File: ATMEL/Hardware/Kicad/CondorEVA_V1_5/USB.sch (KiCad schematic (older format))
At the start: 21 parts, among them J901 USB_2, X901 MINI-USB-32005-201

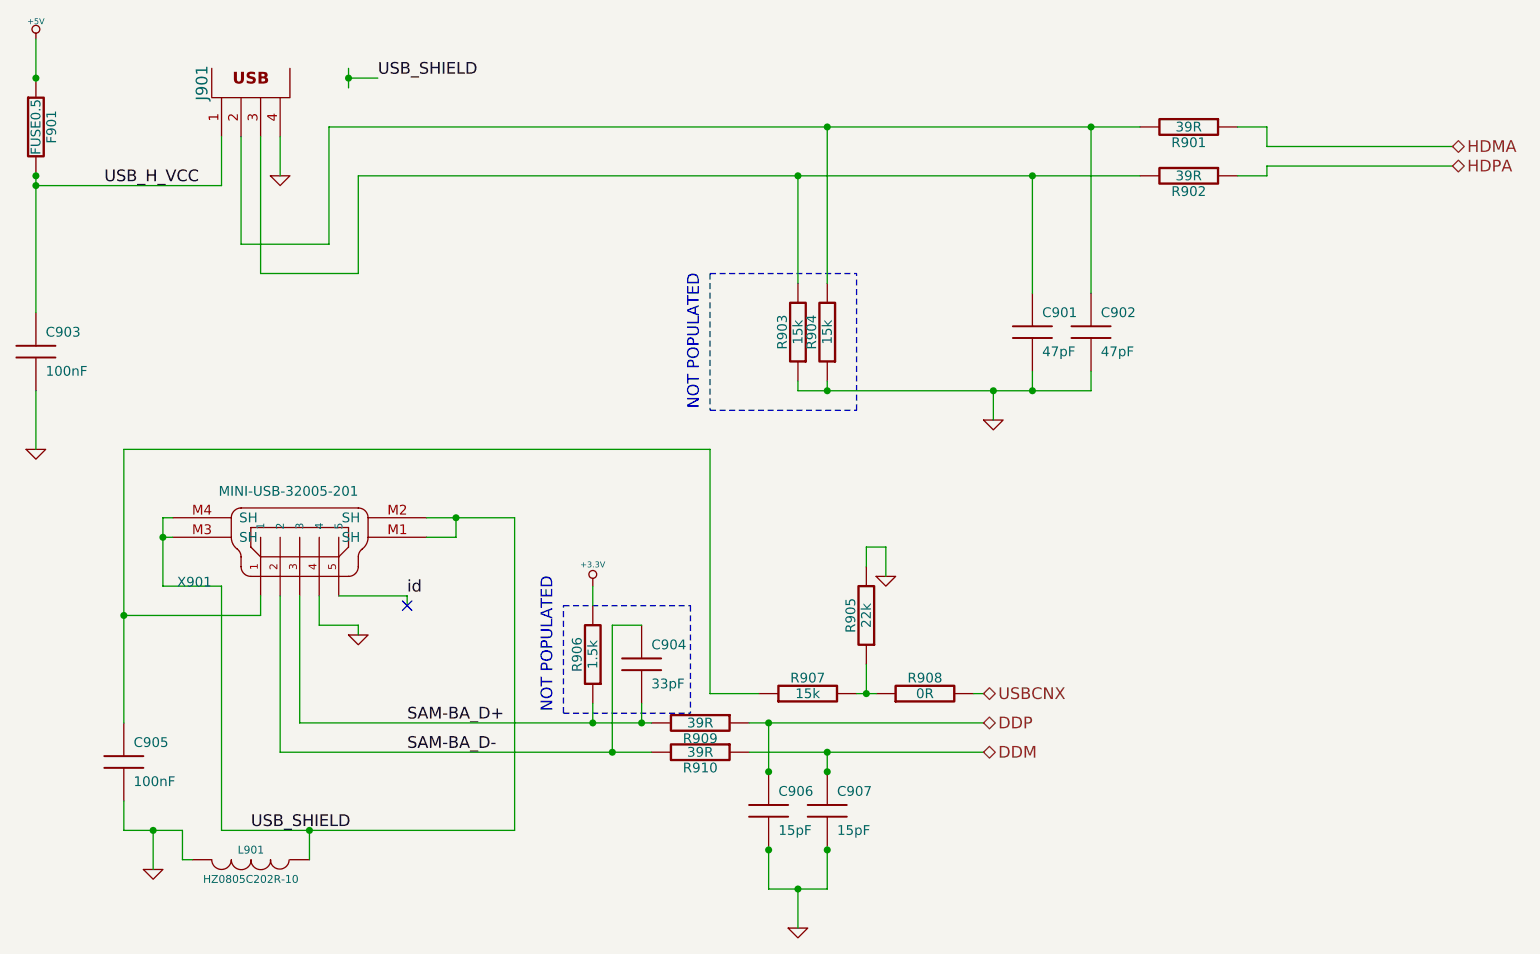
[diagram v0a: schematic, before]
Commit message: Actualización para fabricación lafci Uniandes Enero 19. Orden radicada archivo Ene19.zip con los archivos listos
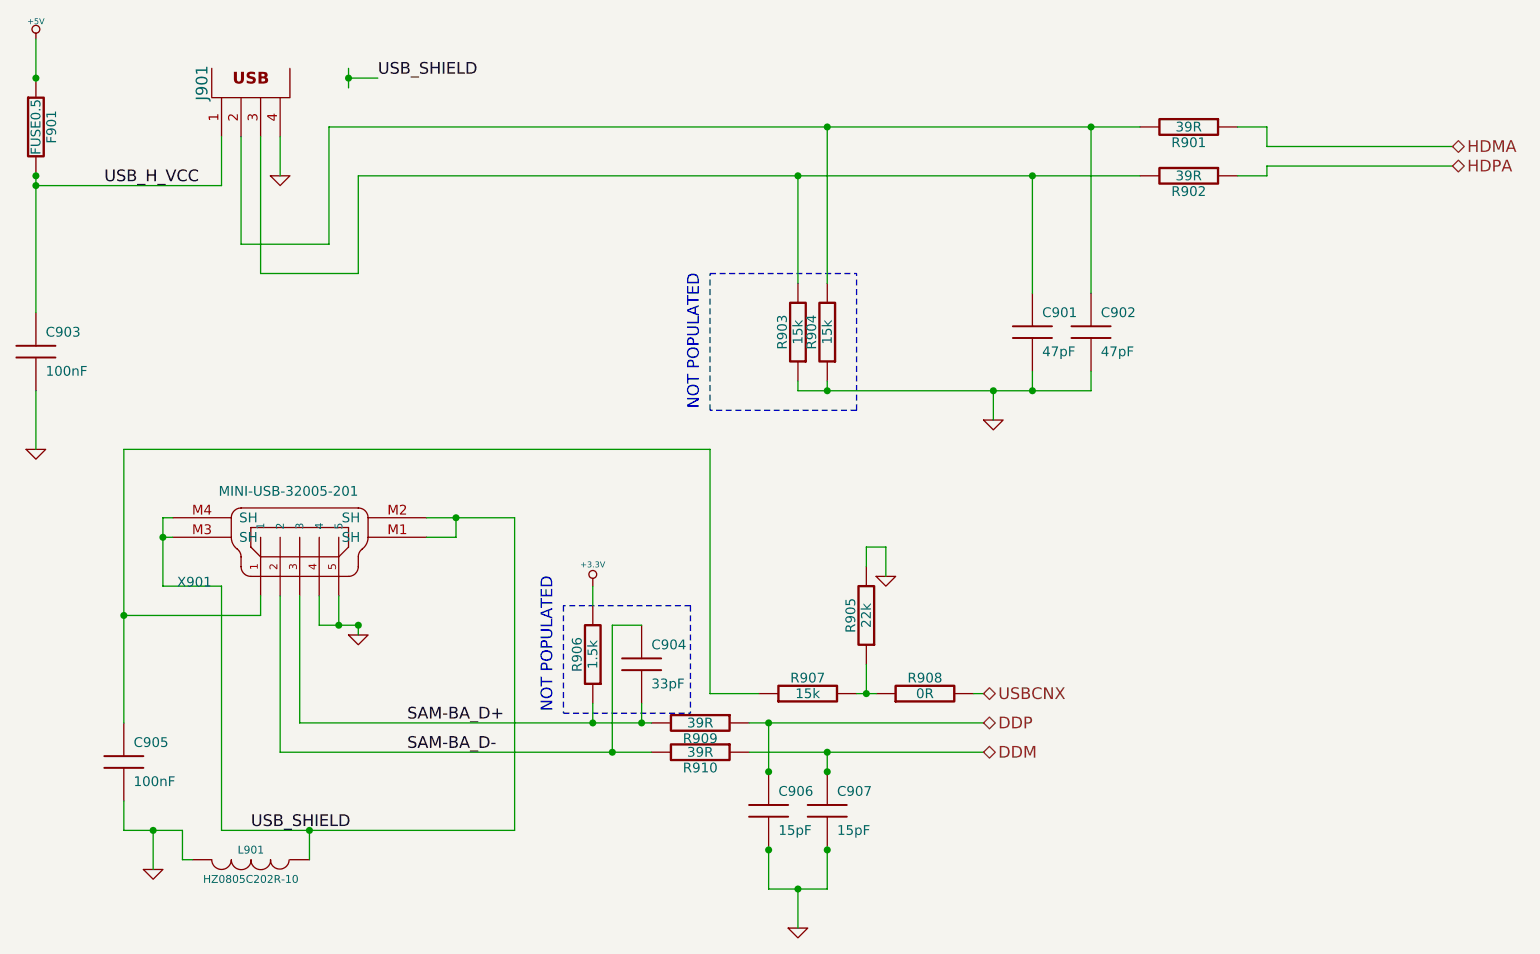
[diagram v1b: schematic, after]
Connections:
- net id is gone; now on net GND: X901.5
- no-connect marks 1 -> 0
